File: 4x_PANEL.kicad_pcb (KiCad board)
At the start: 2 copper layers, 88.4 x 99.2 mm, 8 parts, among them J1 SCART-F, J2 SCART-F

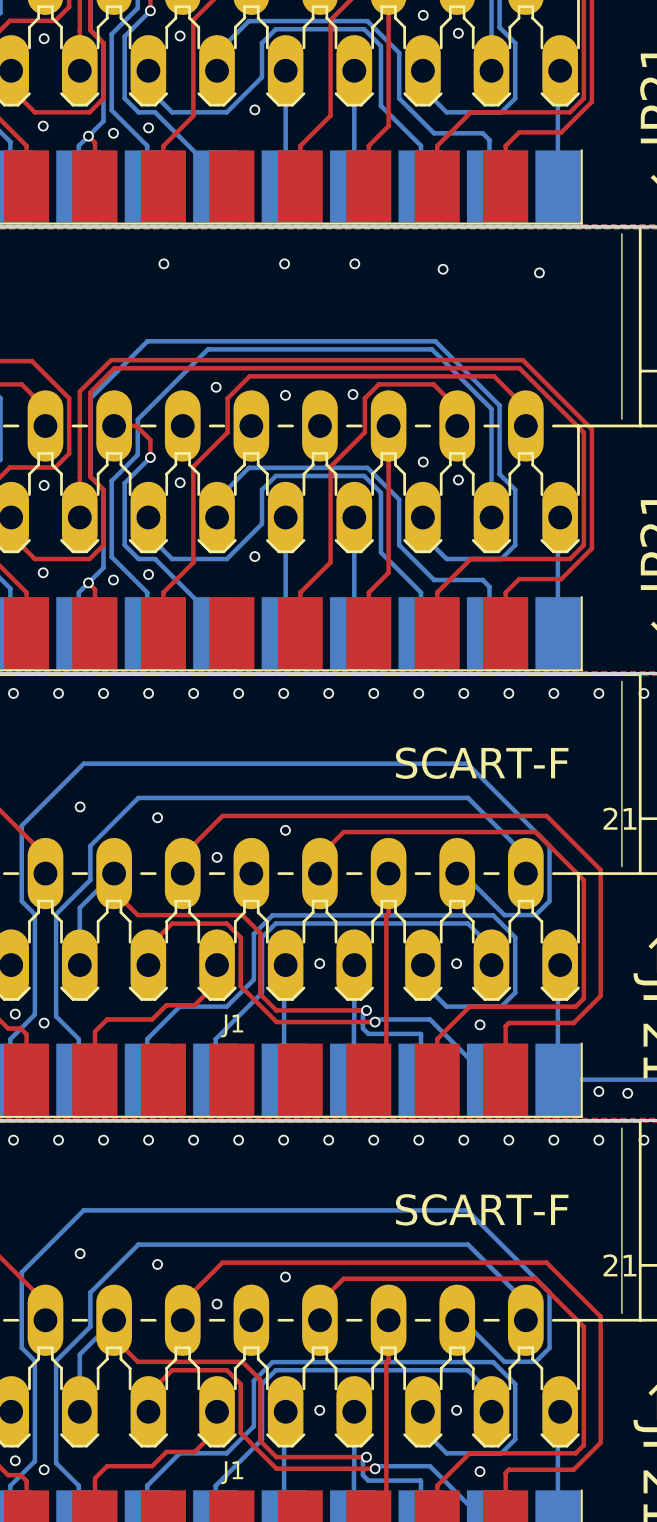
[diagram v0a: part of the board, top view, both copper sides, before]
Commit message: Renamed all gerbers and files to match
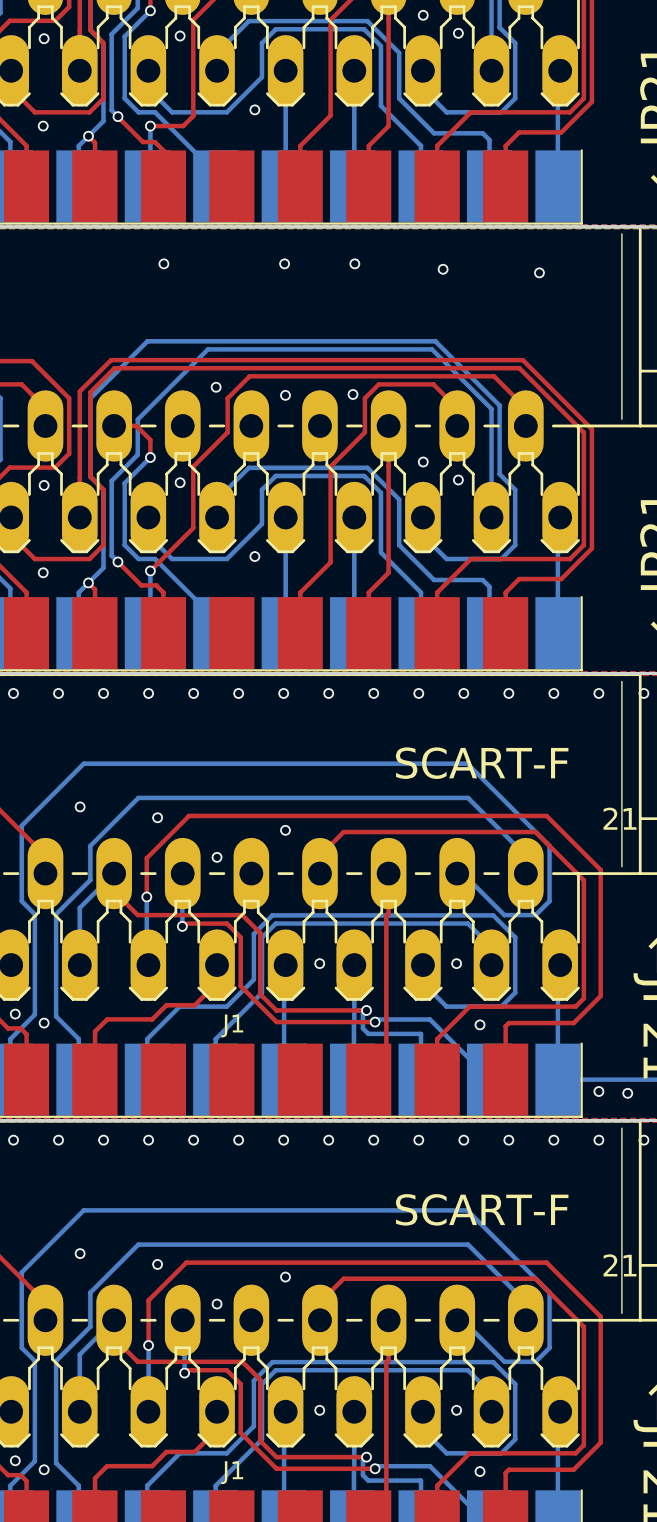
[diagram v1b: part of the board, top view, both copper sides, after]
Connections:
- J2 pad 10: S_IN -> S_OUT (x4)
- J2 pad 9: S_OUT -> S_IN (x4)
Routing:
- net S_IN: track 151.2 -> 167.1 mm, vias 0 -> 4
- net S_OUT: track 137.2 -> 138.0 mm, vias 2 -> 6
- net GND: vias 156 -> 152
